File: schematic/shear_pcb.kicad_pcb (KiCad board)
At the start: 2 copper layers, 71.1 x 76.2 mm, 11 parts, among them J1 MOTOR1, J2 MOTOR2, J3 LCD_CONN, J4 VIN, J5 ENDSTOP1, J6 ENDSTOP2, U1 Teensy3.5, U2 AMIS30542, U3 AMIS30542

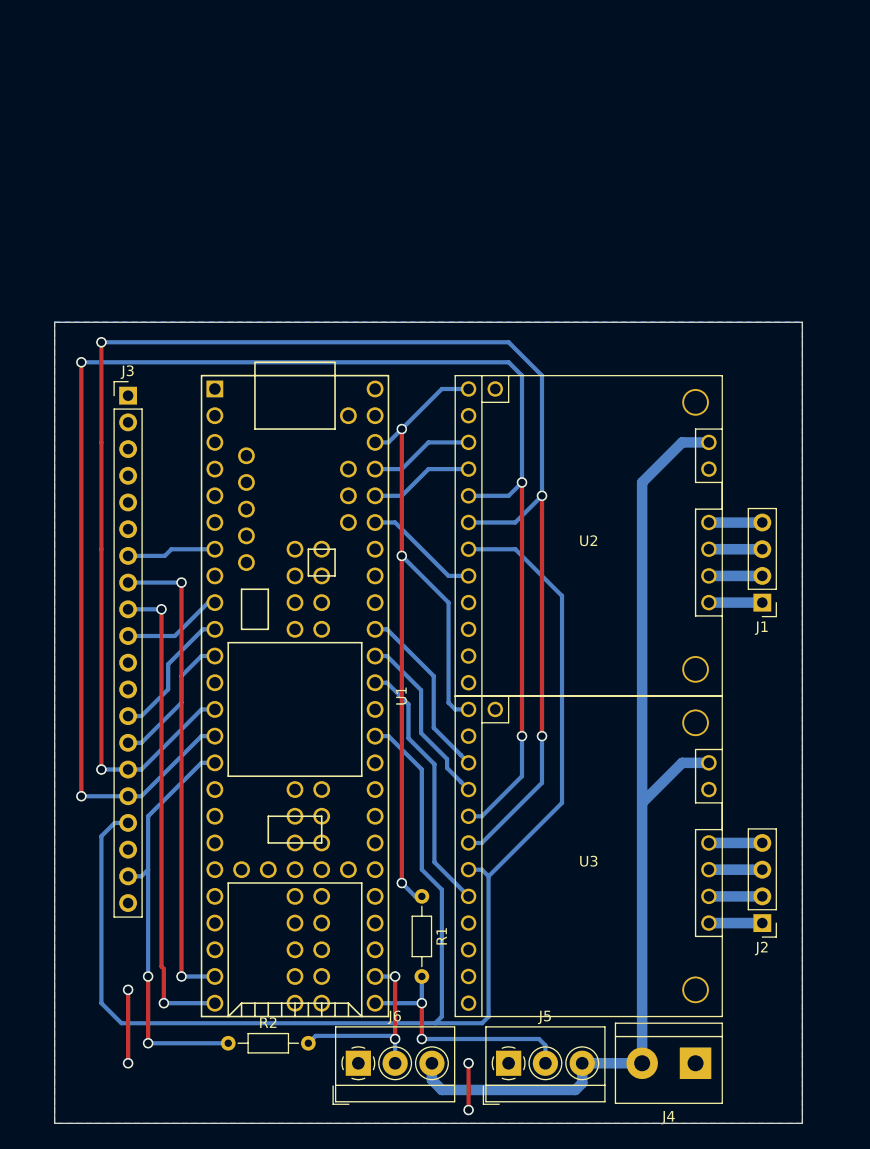
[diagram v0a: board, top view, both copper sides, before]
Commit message: Rework circuit board
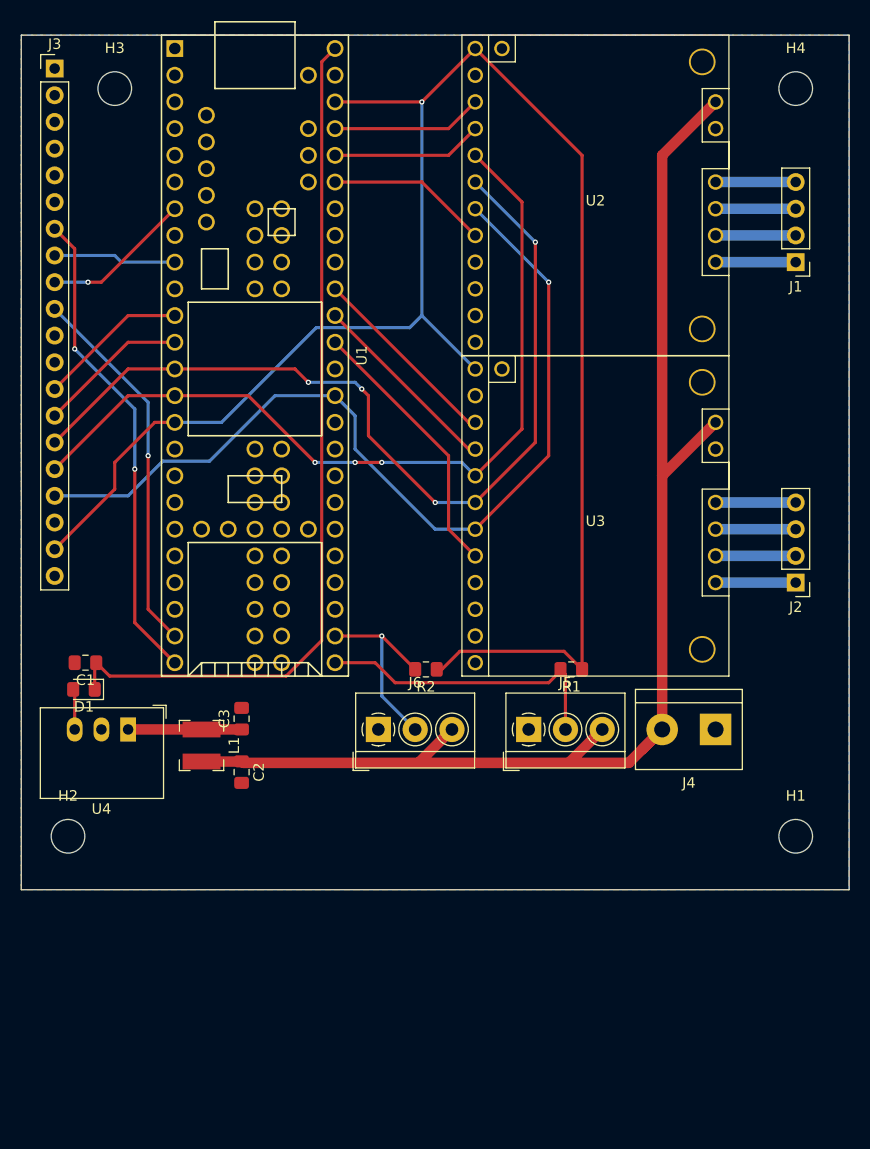
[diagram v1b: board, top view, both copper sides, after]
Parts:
- added C1: 2.2uF, Capacitor_SMD:C_0805_2012Metric_Pad1.15x1.40mm_HandSolder, F.Cu at (124.8, 106.0)
- added C2: 10uF, Capacitor_SMD:C_0805_2012Metric_Pad1.15x1.40mm_HandSolder, F.Cu at (139.7, 116.5)
- added C3: 3.3uF, Capacitor_SMD:C_0805_2012Metric_Pad1.15x1.40mm_HandSolder, F.Cu at (139.7, 111.4)
- added D1: D_Schottky, Diode_SMD:D_0805_2012Metric_Pad1.15x1.40mm_HandSolder, F.Cu at (124.7, 108.6)
- added H1: MountingHole, MountingHole:MountingHole_3.2mm_M3_ISO7380, F.Cu at (192.4, 122.6)
- added H2: MountingHole, MountingHole:MountingHole_3.2mm_M3_ISO7380, F.Cu at (123.2, 122.6)
- added H3: MountingHole, MountingHole:MountingHole_3.2mm_M3_ISO7380, F.Cu at (127.6, 51.4)
- added H4: MountingHole, MountingHole:MountingHole_3.2mm_M3_ISO7380, F.Cu at (192.4, 51.4)
- added L1: 5.6uH, Inductor_SMD:L_Bourns-SRN4018, F.Cu at (135.9, 113.9)
- added U4: R-785.0-1.0, Converter_DCDC:Converter_DCDC_RECOM_R-78E-0.5_THT, F.Cu at (128.9, 112.4)
- R1, R2: footprint Resistor_THT:R_Axial_DIN0204_L3.6mm_D1.6mm_P7.62mm_Horizontal -> Resistor_SMD:R_0805_2012Metric_Pad1.15x1.40mm_HandSolder
- moved R2 40.2 mm to (157.2, 106.7), turned to 180 degrees
- moved U1 32.6 mm to (141.0, 76.8)
- moved J1 32.5 mm to (192.4, 67.9)
- moved J2 32.5 mm to (192.4, 98.4)
- moved U2 32.4 mm to (173.4, 61.6)
- moved U3 32.4 mm to (173.4, 92.1)
- moved J3 31.9 mm to (121.9, 49.5)
- moved J4 31.8 mm to (184.8, 112.4)
- moved J5 31.8 mm to (167.0, 112.4)
- moved J6 31.8 mm to (152.7, 112.4)
- moved R1 25.8 mm to (171.1, 106.7), turned to 180 degrees
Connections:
- J3 pad 1: Net-(J3-Pad1) -> (no net)
- J3 pad 11: Net-(J3-Pad11) -> (no net)
- J3 pad 12: Net-(J3-Pad12) -> (no net)
- J3 pad 18: Net-(J3-Pad18) -> (no net)
- J3 pad 2: Net-(J3-Pad2) -> (no net)
- J3 pad 3: Net-(J3-Pad3) -> (no net)
- J3 pad 4: Net-(J3-Pad4) -> (no net)
- J3 pad 5: Net-(J3-Pad5) -> (no net)
- J3 pad 6: Net-(J3-Pad6) -> (no net)
- U1 pad 10: D\C -> (no net)
- U1 pad 11: CS1 -> D\C
- U1 pad 12: Net-(U1-Pad12) -> CS1
- U1 pad 16: Net-(U1-Pad16) -> (no net)
- U1 pad 17: Net-(U1-Pad17) -> (no net)
- U1 pad 18: Net-(U1-Pad18) -> (no net)
- U1 pad 19: Net-(U1-Pad19) -> (no net)
- U1 pad 2: Net-(U1-Pad2) -> (no net)
- U1 pad 20: Net-(U1-Pad20) -> (no net)
- U1 pad 21: Net-(U1-Pad21) -> (no net)
- U1 pad 22: Net-(U1-Pad22) -> (no net)
- U1 pad 23: YM -> YP
- U1 pad 24: XP -> XM
- U1 pad 25: Net-(U1-Pad25) -> (no net)
- U1 pad 26: Net-(U1-Pad26) -> (no net)
- U1 pad 27: Net-(U1-Pad27) -> (no net)
- U1 pad 28: Net-(U1-Pad28) -> (no net)
- U1 pad 29: Net-(U1-Pad29) -> (no net)
- U1 pad 3: Net-(U1-Pad3) -> (no net)
- U1 pad 32: Net-(U1-Pad32) -> (no net)
- U1 pad 33: Net-(U1-Pad33) -> (no net)
- U1 pad 34: Net-(U1-Pad34) -> (no net)
- U1 pad 35: Net-(U1-Pad35) -> (no net)
- U1 pad 36: Net-(U1-Pad36) -> (no net)
- U1 pad 37: Net-(U1-Pad37) -> (no net)
- U1 pad 38: Net-(U1-Pad38) -> (no net)
- U1 pad 39: Net-(U1-Pad39) -> (no net)
- U1 pad 4: Net-(U1-Pad4) -> (no net)
- U1 pad 41: Net-(U1-Pad41) -> (no net)
- U1 pad 45: Net-(U1-Pad45) -> (no net)
- U1 pad 46: Net-(U1-Pad46) -> (no net)
- U1 pad 47: Net-(U1-Pad47) -> (no net)
- U1 pad 5: Net-(U1-Pad5) -> (no net)
- U1 pad 52: Net-(U1-Pad52) -> (no net)
- U1 pad 53: Net-(U1-Pad53) -> +5V
- U1 pad 54: Net-(U1-Pad54) -> (no net)
- U1 pad 55: Net-(U1-Pad55) -> (no net)
- U1 pad 56: Net-(U1-Pad56) -> (no net)
- U1 pad 57: Net-(U1-Pad57) -> (no net)
- U1 pad 58: Net-(U1-Pad58) -> (no net)
- U1 pad 59: Net-(U1-Pad59) -> (no net)
- U1 pad 6: Net-(U1-Pad6) -> (no net)
- U1 pad 60: Net-(U1-Pad60) -> (no net)
- U1 pad 61: Net-(U1-Pad61) -> (no net)
- U1 pad 62: Net-(U1-Pad62) -> (no net)
- U1 pad 63: Net-(U1-Pad63) -> (no net)
- U1 pad 64: Net-(U1-Pad64) -> (no net)
- U1 pad 65: Net-(U1-Pad65) -> (no net)
- U1 pad 66: Net-(U1-Pad66) -> (no net)
- U1 pad 67: Net-(U1-Pad67) -> (no net)
- U1 pad 68: Net-(U1-Pad68) -> (no net)
- U1 pad 69: Net-(U1-Pad69) -> (no net)
- U1 pad 7: XM -> XP
- U1 pad 70: Net-(U1-Pad70) -> (no net)
- U1 pad 71: Net-(U1-Pad71) -> (no net)
- U1 pad 72: Net-(U1-Pad72) -> (no net)
- U1 pad 73: Net-(U1-Pad73) -> (no net)
- U1 pad 74: Net-(U1-Pad74) -> (no net)
- U1 pad 75: Net-(U1-Pad75) -> (no net)
- U1 pad 76: Net-(U1-Pad76) -> (no net)
- U1 pad 77: Net-(U1-Pad77) -> (no net)
- U1 pad 78: Net-(U1-Pad78) -> (no net)
- U1 pad 79: Net-(U1-Pad79) -> (no net)
- U1 pad 8: Net-(U1-Pad8) -> (no net)
- U1 pad 80: Net-(U1-Pad80) -> (no net)
- U1 pad 81: Net-(U1-Pad81) -> (no net)
- U1 pad 82: Net-(U1-Pad82) -> (no net)
- U1 pad 83: Net-(U1-Pad83) -> (no net)
- U1 pad 84: Net-(U1-Pad84) -> (no net)
- U1 pad 85: Net-(U1-Pad85) -> (no net)
- U1 pad 86: Net-(U1-Pad86) -> (no net)
- U1 pad 9: YP -> YM
- U2 pad 1: Net-(U2-Pad1) -> (no net)
- U2 pad 10: Net-(U2-Pad10) -> (no net)
- U2 pad 11: Net-(U2-Pad11) -> (no net)
- U2 pad 12: Net-(U2-Pad12) -> (no net)
- U2 pad 13: Net-(U2-Pad13) -> (no net)
- U2 pad 3: Net-(U2-Pad3) -> GND
- U3 pad 1: Net-(U3-Pad1) -> (no net)
- U3 pad 10: Net-(U3-Pad10) -> (no net)
- U3 pad 11: Net-(U3-Pad11) -> (no net)
- U3 pad 12: Net-(U3-Pad12) -> (no net)
- U3 pad 13: Net-(U3-Pad13) -> (no net)
- U3 pad 3: Net-(U3-Pad3) -> GND
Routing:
- net +5V: track 0.00 -> 82.6 mm
- net MISO: track 149.1 -> 80.2 mm, vias 4 -> 3
- net MOSI: track 153.2 -> 85.6 mm
- net CLK: track 143.6 -> 87.3 mm, vias 0 -> 1
- net +3V3: track 114.4 -> 167.1 mm, vias 5 -> 1
- net XM: track 8.52 -> 46.0 mm, vias 0 -> 2
- net YM: track 45.7 -> 11.7 mm, vias 2 -> 0
- net XP: track 45.6 -> 14.3 mm, vias 2 -> 1
- net VDC: track 95.2 -> 125.9 mm
- net YP: track 9.57 -> 35.8 mm, vias 0 -> 1
- net GND: track 11.4 -> 0.00 mm, vias 4 -> 0
- net Net-(C3-Pad1): track 0.00 -> 10.8 mm
- net END1: track 24.3 -> 28.8 mm, vias 2 -> 0
- net STEP1: track 9.94 -> 14.4 mm
- net DIR1: track 9.94 -> 14.4 mm
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- added copper zone on F.Cu, net GND
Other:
- board size 71.1 x 76.2 mm -> 78.7 x 81.3 mm
- net class Default: clearance 0.8 -> 0.2; trace_width 0.4 -> 0.3; via_dia 1 -> 0.5; via_drill 0.7 -> 0.25
- net class Motor: clearance 0.8 -> 0.2; via_dia 1 -> 1.2; via_drill 0.7 -> 0.8
- net class Power: clearance 0.8 -> 0.2; via_dia 1 -> 1.2; via_drill 0.7 -> 0.8
- rule trace_clearance: 0.8 -> 0.2
- rule trace_min: 0.4 -> 0.3
- rule via_min_drill: 0.7 -> 0.2
- rule via_min_size: 1 -> 0.5
